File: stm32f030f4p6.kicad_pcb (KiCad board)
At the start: 2 copper layers, 16.8 x 65.5 mm, 13 parts, among them P1 BOOT, P2 CONF, P3 LEFT_PINOUT, P4 RIGHT_PINOUT, P5 SWD, P6 VCC, SW1 RESET, U1 AP1117D33, U2 STM32F030F4

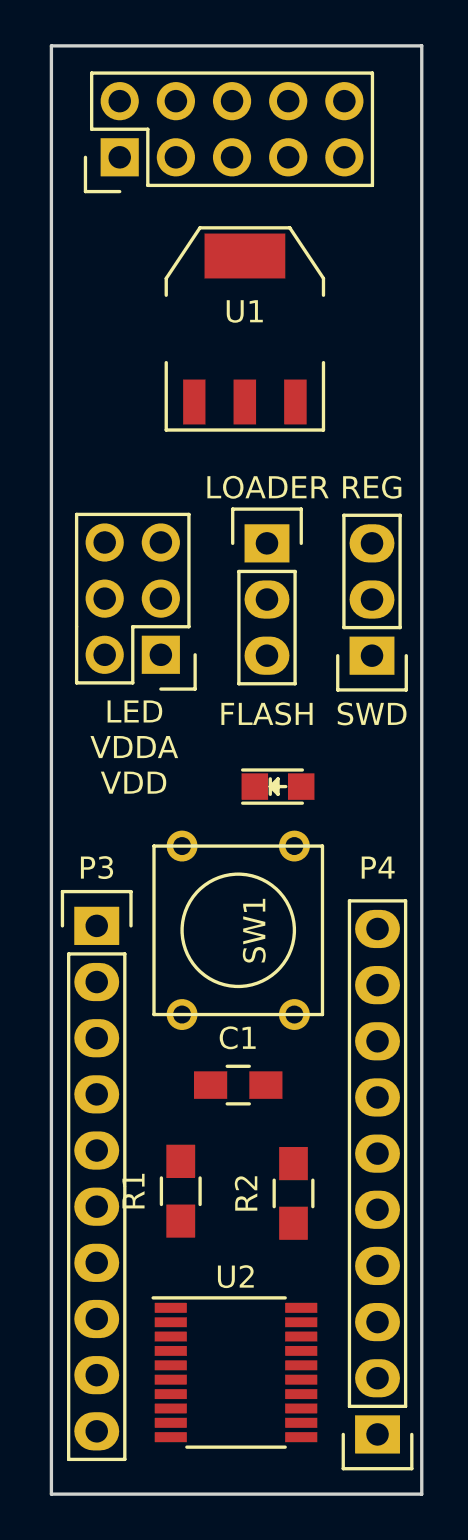
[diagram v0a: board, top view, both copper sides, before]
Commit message: shrinkify.
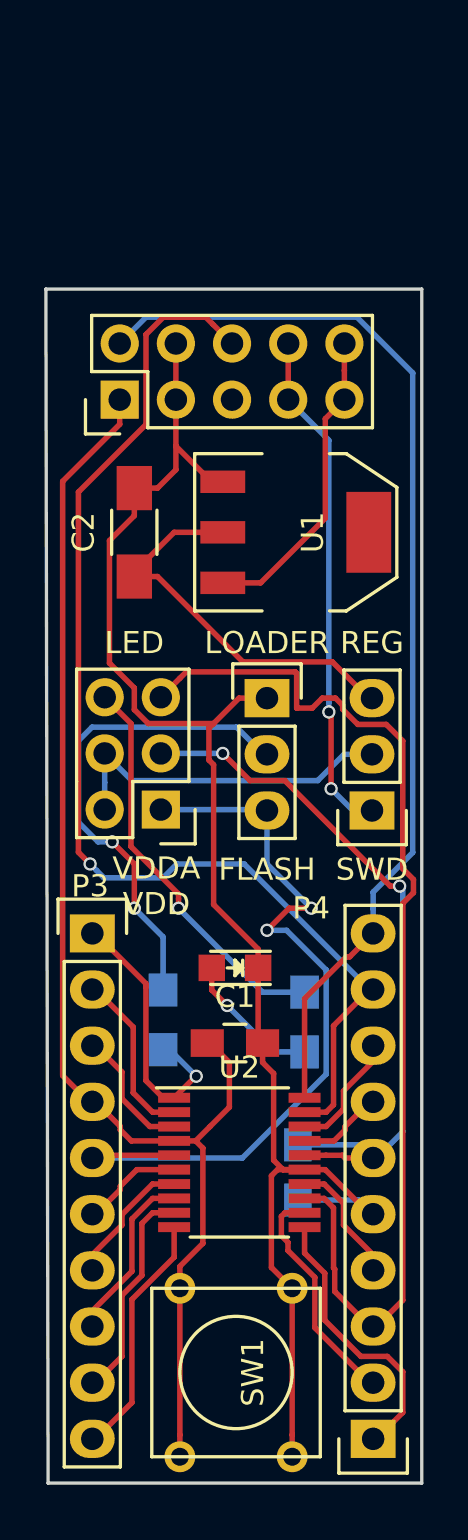
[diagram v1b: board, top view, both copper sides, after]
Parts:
- added C2: 10uF, Capacitors_SMD:C_1206_HandSoldering, F.Cu at (148.0, 114.0)
- added C3: C, Capacitors_SMD:C_0805_HandSoldering, B.Cu at (155.4, 142.9)
- R1, R2: moved to B.Cu
- moved SW1 20.0 mm to (152.6, 152.0)
- moved P5 11.0 mm to (147.3, 108.0)
- moved U2 9.50 mm to (152.8, 142.5)
- moved U1 9.48 mm to (155.3, 114.0), turned to 270 degrees
- moved D1 8.43 mm to (152.6, 133.7), turned to 180 degrees
- moved R1 7.79 mm to (149.3, 136.1)
- moved R2 7.77 mm to (155.7, 136.2)
- moved P1 7.00 mm to (154.0, 121.5)
- moved P2 7.00 mm to (149.2, 126.5)
- moved P6 7.00 mm to (158.8, 126.6)
- moved C1 1.91 mm to (152.6, 137.1)
- moved P3 0.39 mm to (146.1, 132.1)
- moved P4 0.28 mm to (158.8, 155.0)
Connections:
- P5 pad 1: VSS -> NRST
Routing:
- net VSS: track 0.00 -> 74.8 mm
- net NRST: track 0.00 -> 59.5 mm
- net PA13: track 0.00 -> 53.3 mm, vias 0 -> 1
- net PA14: track 0.00 -> 49.8 mm
- net PA7: track 0.00 -> 49.3 mm
- net VDDA: track 0.00 -> 36.9 mm, vias 0 -> 3
- net VDD: track 0.00 -> 34.4 mm, vias 0 -> 2
- net SWD_3.3V: track 0.00 -> 23.2 mm, vias 0 -> 2
- net Net-(P1-Pad2): track 0.00 -> 22.7 mm, vias 0 -> 2
- net Net-(P2-Pad6): track 0.00 -> 18.2 mm, vias 0 -> 1
- net REG_3.3V: track 0.00 -> 18.1 mm
- net Net-(P2-Pad2): track 0.00 -> 15.6 mm
- net SWD_5V: track 0.00 -> 14.1 mm
- net BOOT0: track 0.00 -> 13.0 mm, vias 0 -> 1
- net PA5: track 0.00 -> 12.8 mm
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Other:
- board size 16.8 x 65.5 mm -> 17 x 54 mm
- board text added: "LED"
- board text added: "VDDA VDD"
- board text removed: "LED VDDA VDD"
